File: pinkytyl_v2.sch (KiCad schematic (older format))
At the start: 58 parts, among them J1 STX-3501-3N, J2 Conn_01x02, J3 USB_B_Mini, J5 Conn_02x05_Odd_Even, K0 KEYSW, K10 KEYSW, K11 KEYSW, K12 KEYSW, K13 KEYSW, K14 KEYSW, K15 KEYSW, K20 KEYSW, K21 KEYSW, K22 KEYSW, K23 KEYSW, K24 KEYSW, K25 KEYSW, K30 KEYSW, K31 KEYSW, K32 KEYSW, K33 KEYSW, K34 KEYSW, K35 KEYSW, K40 KEYSW, K41 KEYSW, U1 ATmega32U4-MU, Y1 Crystal_GND24_Small

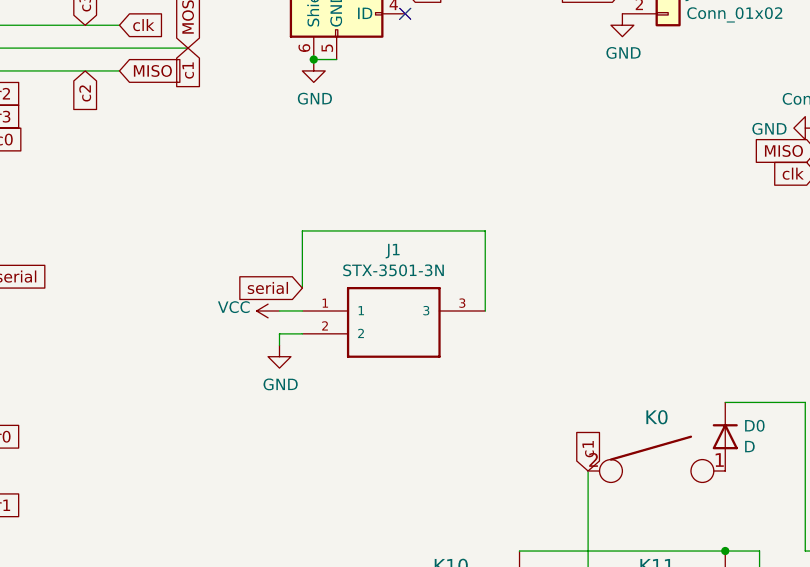
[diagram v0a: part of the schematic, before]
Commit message: In the middle of slim redesign
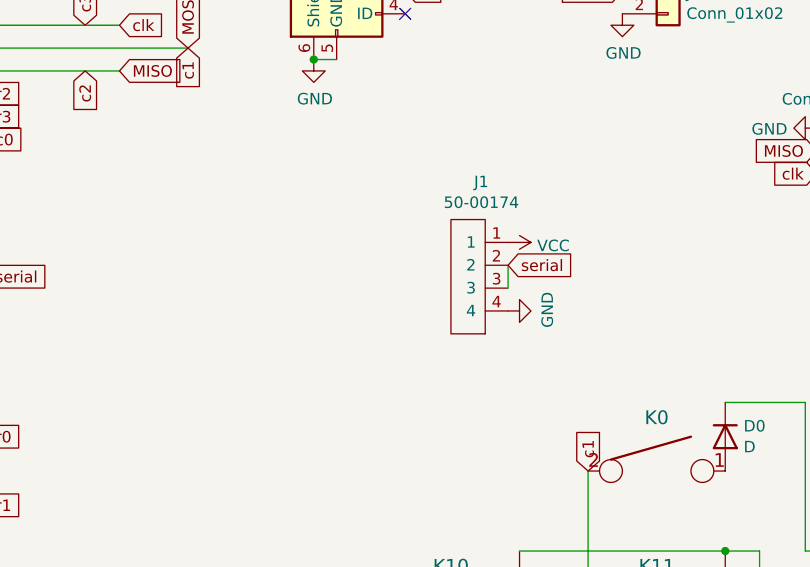
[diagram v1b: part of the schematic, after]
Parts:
- removed J1: STX-3501-3N, STX-3501-3N:STX35013N, symbol STX-3501-3N:STX-3501-3N
- added J1: 50-00174, misc:54-00174, symbol misc:50-00174
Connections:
- net GND: now also J1.4
- net VCC: now also J1.1
- net serial: now also J1.2, J1.3
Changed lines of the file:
@@
 	1    0    0    -1
 $EndComp
-Text GLabel 4900 2450 0    50   Input ~ 0
+Text GLabel 5800 2350 2    50   Input ~ 0
 serial
 $Comp
 L power:VCC #PWR0114
 U 1 1 614F8A38
-P 4800 2550
-F 0 "#PWR0114" H 4800 2400 50  0001 C CNN
-F 1 "VCC" V 4815 2677 50  0000 L CNN
-F 2 "" H 4800 2550 50  0001 C CNN
-F 3 "" H 4800 2550 50  0001 C CNN
-	1    4800 2550
-	0    -1   -1   0
+P 5800 2250
+F 0 "#PWR0114" H 5800 2100 50  0001 C CNN
+F 1 "VCC" V 5815 2377 50  0000 L CNN
+F 2 "" H 5800 2250 50  0001 C CNN
+F 3 "" H 5800 2250 50  0001 C CNN
+	1    5800 2250
+	0    1    1    0
 $EndComp
 $Comp
 L power:GND #PWR0113
 U 1 1 614F8A30
-P 4800 2700
-F 0 "#PWR0113" H 4800 2450 50  0001 C CNN
-F 1 "GND" H 4805 2527 50  0000 C CNN
-F 2 "" H 4800 2700 50  0001 C CNN
-F 3 "" H 4800 2700 50  0001 C CNN
-	1    4800 2700
-	1    0    0    -1
+P 5800 2550
+F 0 "#PWR0113" H 5800 2300 50  0001 C CNN
+F 1 "GND" H 5805 2377 50  0000 C CNN
+F 2 "" H 5800 2550 50  0001 C CNN
+F 3 "" H 5800 2550 50  0001 C CNN
+	1    5800 2550
+	0    -1   -1   0
 $EndComp
 Text GLabel 5350 1150 2    50   Input ~ 0
@@
 	2200 1200 2150 1200
 Wire Wire Line
-	4900 2550 4800 2550
-Wire Wire Line
-	4800 2650 4800 2700
-Wire Wire Line
-	4900 2650 4800 2650
-Wire Wire Line
 	5050 1450 4950 1450
 Connection ~ 4950 1450
@@
 Connection ~ 2100 1300
 $Comp
-L STX-3501-3N:STX-3501-3N J1
-U 1 1 615C1FA9
-P 4900 2550
-F 0 "J1" H 5300 2817 50  0000 C CNN
-F 1 "STX-3501-3N" H 5300 2726 50  0000 C CNN
-F 2 "STX-3501-3N:STX35013N" H 4900 2550 50  0001 L BNN
-F 3 "" H 4900 2550 50  0001 L BNN
-F 4 "Kycon, Inc." H 4900 2550 50  0001 L BNN "Manufacturer_Name"
-F 5 "" H 4900 2550 50  0001 L BNN "Arrow_Price-Stock"
-F 6 "STX-3501-3N" H 4900 2550 50  0001 L BNN "Manufacturer_Part_Number"
-F 7 "" H 4900 2550 50  0001 L BNN "Arrow_Part_Number"
-F 8 "Phone Connectors 3.5mm S LUGS STEREO 3P THRU HOLE" H 4900 2550 50  0001 L BNN "Description"
-F 9 "5mm" H 4900 2550 50  0001 L BNN "Height"
-F 10 "" H 4900 2550 50  0001 L BNN "Mouser_Price-Stock"
-F 11 "" H 4900 2550 50  0001 L BNN "Mouser_Part_Number"
-	1    4900 2550
-	1    0    0    -1
-$EndComp
-Wire Wire Line
-	5700 2550 5700 2200
-Wire Wire Line
-	5700 2200 4900 2200
-Wire Wire Line
-	4900 2200 4900 2450
-$Comp
 L Connector_Generic:Conn_01x02 J2
 U 1 1 615E9C63
@@
 Text GLabel 6300 1150 0    50   Input ~ 0
 reset
+$Comp
+L misc:50-00174 J1
+U 1 1 614D3F66
+P 5800 2100
+F 0 "J1" H 5683 2215 50  0000 C CNN
+F 1 "50-00174" H 5683 2124 50  0000 C CNN
+F 2 "misc:54-00174" H 5800 2100 50  0001 C CNN
+F 3 "" H 5800 2100 50  0001 C CNN
+	1    5800 2100
+	1    0    0    -1
+$EndComp
+Wire Wire Line
+	5800 2450 5800 2350
 $EndSCHEMATC
